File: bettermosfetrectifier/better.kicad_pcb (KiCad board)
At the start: 2 copper layers, 42 parts, among them IC1 LT4322RMS8#PBF, IC2 LT4322RMS8#PBF, IC3 LT4322RMS8#PBF, IC4 LT4322RMS8#PBF, IC5 LT4322RMS8#PBF, IC6 LT4322RMS8#PBF, J1 Conn_01x02, J2 Conn_01x03, Q10 DN3135, Q11 DN3135, Q12 DN3135, Q13 BSC050N10NS5ATMA1, Q14 BSC050N10NS5ATMA1, Q16 BSC050N10NS5ATMA1, Q17 BSC050N10NS5ATMA1, Q18 BSC050N10NS5ATMA1, Q19 BSC050N10NS5ATMA1, Q7 DN3135, Q8 DN3135, Q9 DN3135

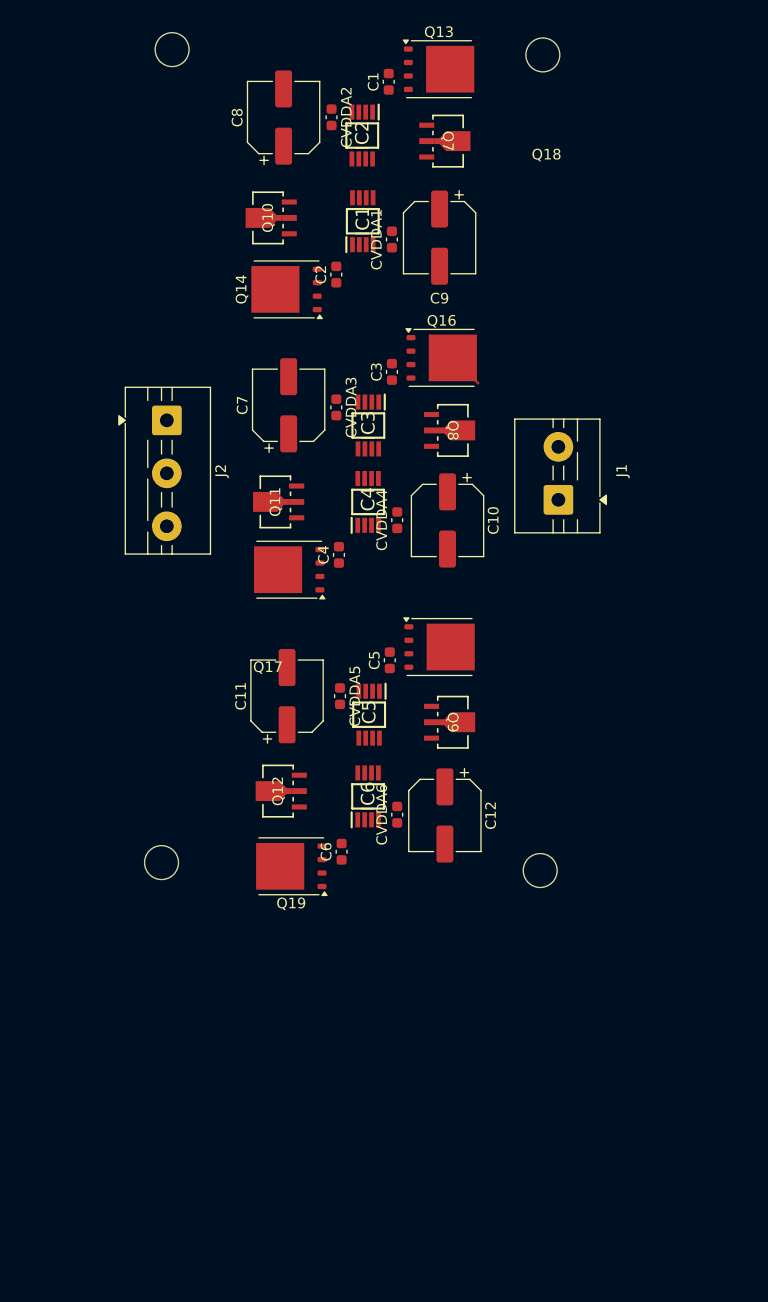
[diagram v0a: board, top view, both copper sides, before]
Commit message: idk improved layout a bit
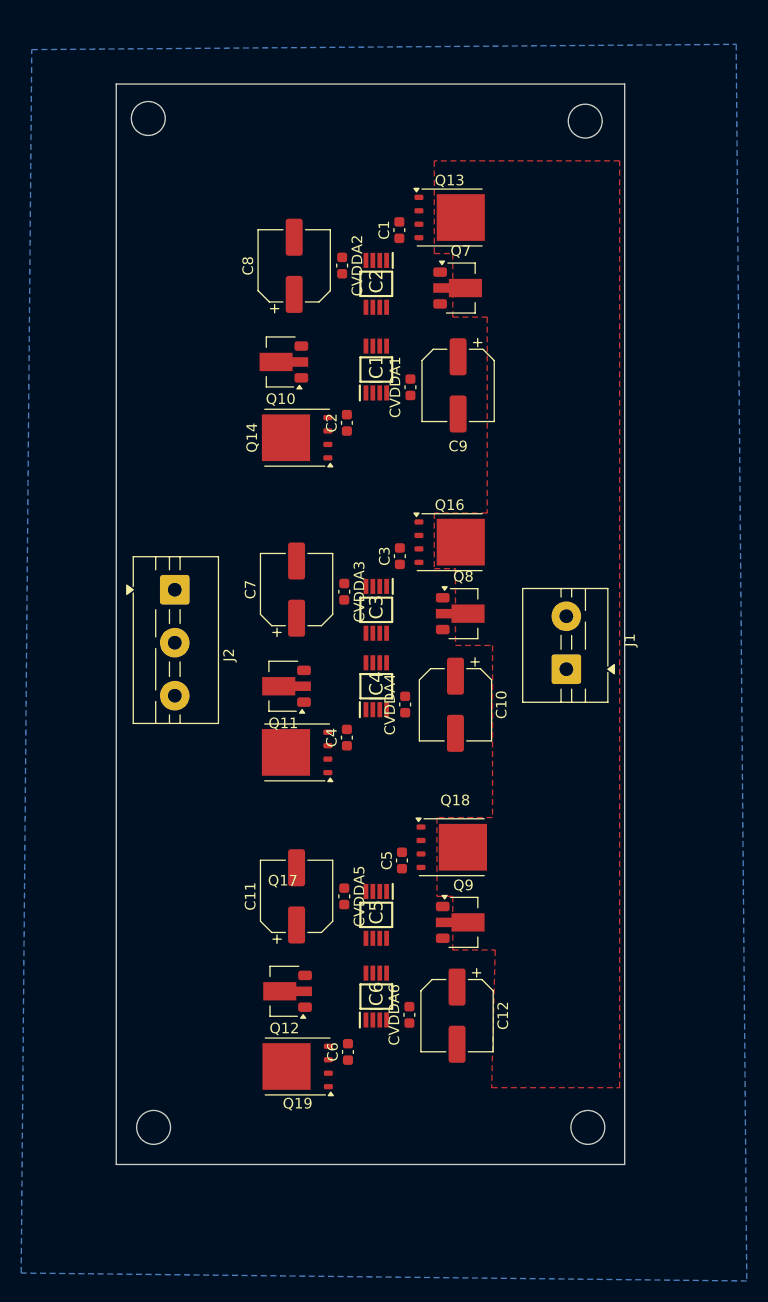
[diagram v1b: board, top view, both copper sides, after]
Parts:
- Q10, Q11, Q12, Q7, Q8, Q9: footprint Library:SOT-89_3MC_MCH -> Package_TO_SOT_SMD:SOT-89-3
- moved H2 25.0 mm to (155.8, 118.0)
- moved H1 24.7 mm to (196.8, 118.0)
- moved C12 18.9 mm to (184.4, 107.5)
- moved CVDDA6 18.9 mm to (179.9, 107.4)
- moved Q18 18.9 mm to (183.9, 91.5)
- moved C5 18.9 mm to (179.2, 92.8)
- moved Q9 18.9 mm to (185.0, 98.6), turned to 0 degrees
- moved C11 18.9 mm to (169.2, 96.2)
- moved IC6 18.9 mm to (176.8, 105.7)
- moved IC5 18.9 mm to (176.8, 97.9)
- moved C6 18.9 mm to (174.1, 110.9)
- moved Q12 18.9 mm to (168.1, 105.2), turned to 180 degrees
- moved Q19 18.9 mm to (169.3, 112.2)
- moved CVDDA5 18.9 mm to (173.8, 96.2)
- moved IC4 17.4 mm to (176.8, 76.3)
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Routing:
- net Net-(J1-Pin_1): track 3.41 -> 0.00 mm
- added copper zone on B.Cu, net GND
- added copper zone on F.Cu, net Net-(J1-Pin_1)
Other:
- board outline added: 48 x 102 mm
